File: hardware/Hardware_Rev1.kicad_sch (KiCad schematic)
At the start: 150 parts, among them J1 RJ45_LED_Shielded, Q1 BSS138, Q10 Q_PMOS_GSD, Q11 Q_PMOS_GSD, Q12 Q_PMOS_GSD, Q13 BSS138, Q14 BSS138, Q15 BSS138, Q16 Q_PMOS_GSD, Q17 Q_PMOS_GSD, Q18 Q_PMOS_GSD, Q19 BSS138, Q2 BSS138, Q20 BSS138, Q21 BSS138, Q22 Q_PMOS_GSD, Q23 Q_PMOS_GSD, Q24 Q_PMOS_GSD, Q3 BSS138, Q4 Q_PMOS_GSD, Q5 Q_PMOS_GSD, Q6 Q_PMOS_GSD, Q7 BSS138, Q8 BSS138, Q9 BSS138, U1 OKI, U2 Teensy4.1_DEV-16771

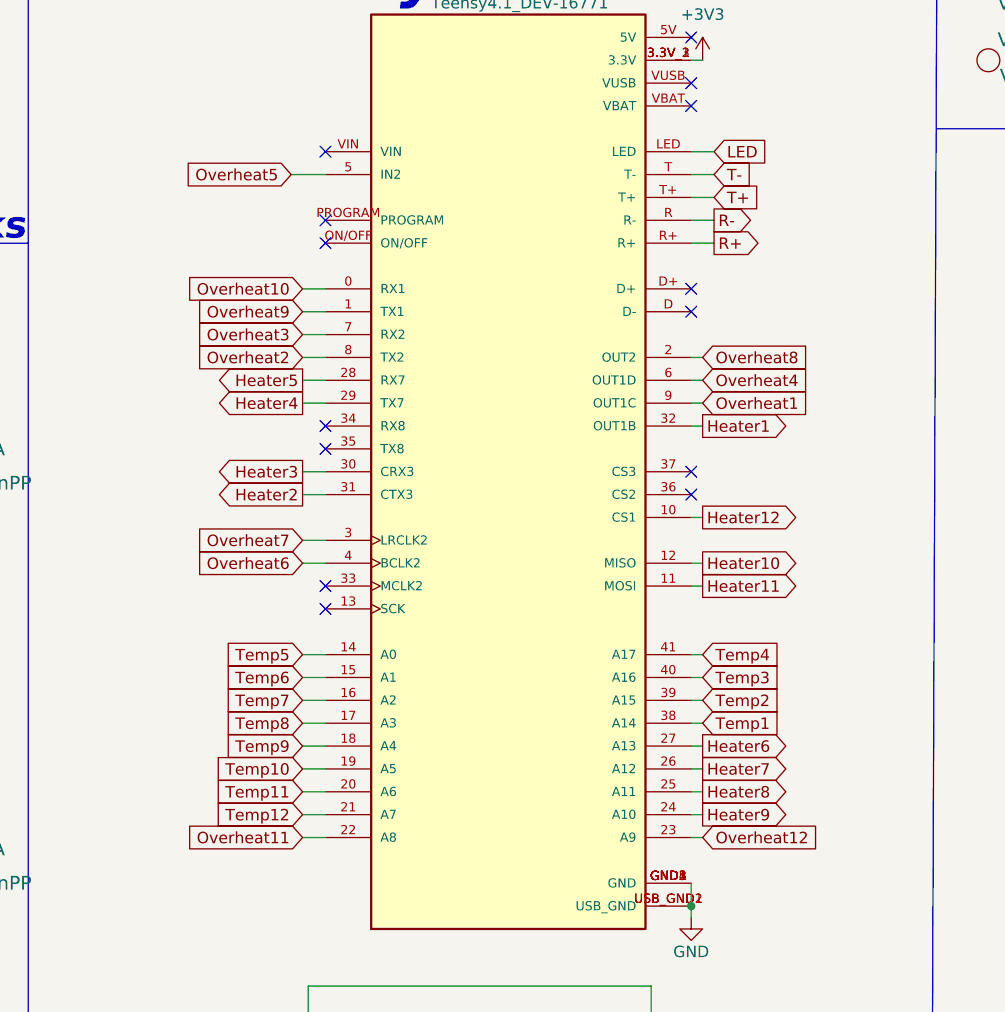
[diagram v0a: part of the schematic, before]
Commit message: Finished components + Traces
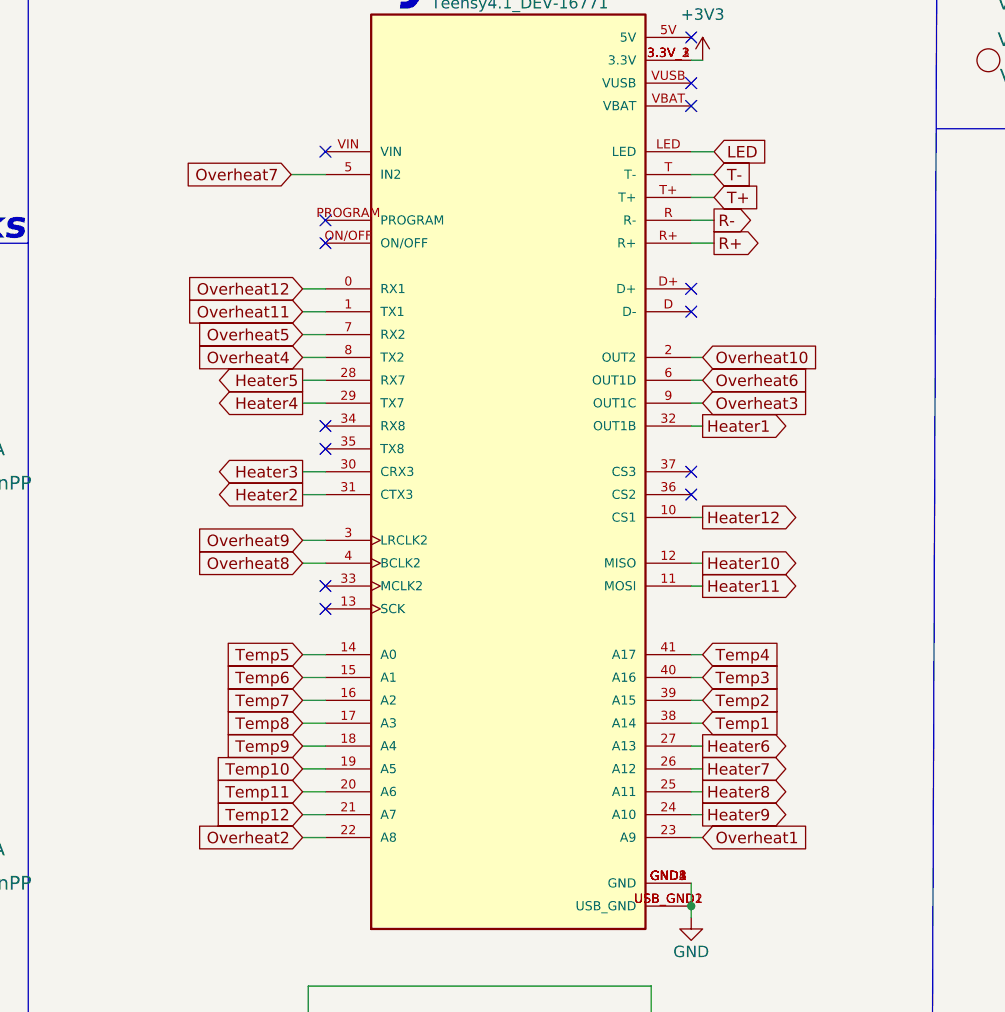
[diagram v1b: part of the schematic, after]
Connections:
- net Overheat1: now also U2.23 (A9); no longer U2.9 (OUT1C)
- net Overheat10: now also U2.2 (OUT2); no longer U2.0 (RX1)
- net Overheat11: now also U2.1 (TX1); no longer U2.22 (A8)
- net Overheat12: now also U2.0 (RX1); no longer U2.23 (A9)
- net Overheat2: now also U2.22 (A8); no longer U2.8 (TX2)
- net Overheat3: now also U2.9 (OUT1C); no longer U2.7 (RX2)
- net Overheat4: now also U2.8 (TX2); no longer U2.6 (OUT1D)
- net Overheat5: now also U2.7 (RX2); no longer U2.5 (IN2)
- net Overheat6: now also U2.6 (OUT1D); no longer U2.4 (BCLK2)
- net Overheat7: now also U2.5 (IN2); no longer U2.3 (LRCLK2)
- net Overheat8: now also U2.4 (BCLK2); no longer U2.2 (OUT2)
- net Overheat9: now also U2.3 (LRCLK2); no longer U2.1 (TX1)
